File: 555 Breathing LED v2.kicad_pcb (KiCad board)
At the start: 2 copper layers, 80.8 x 35.6 mm, 17 parts, among them Q1 PN2222A, SW1 SW_SPDT, U1 LMC555xN

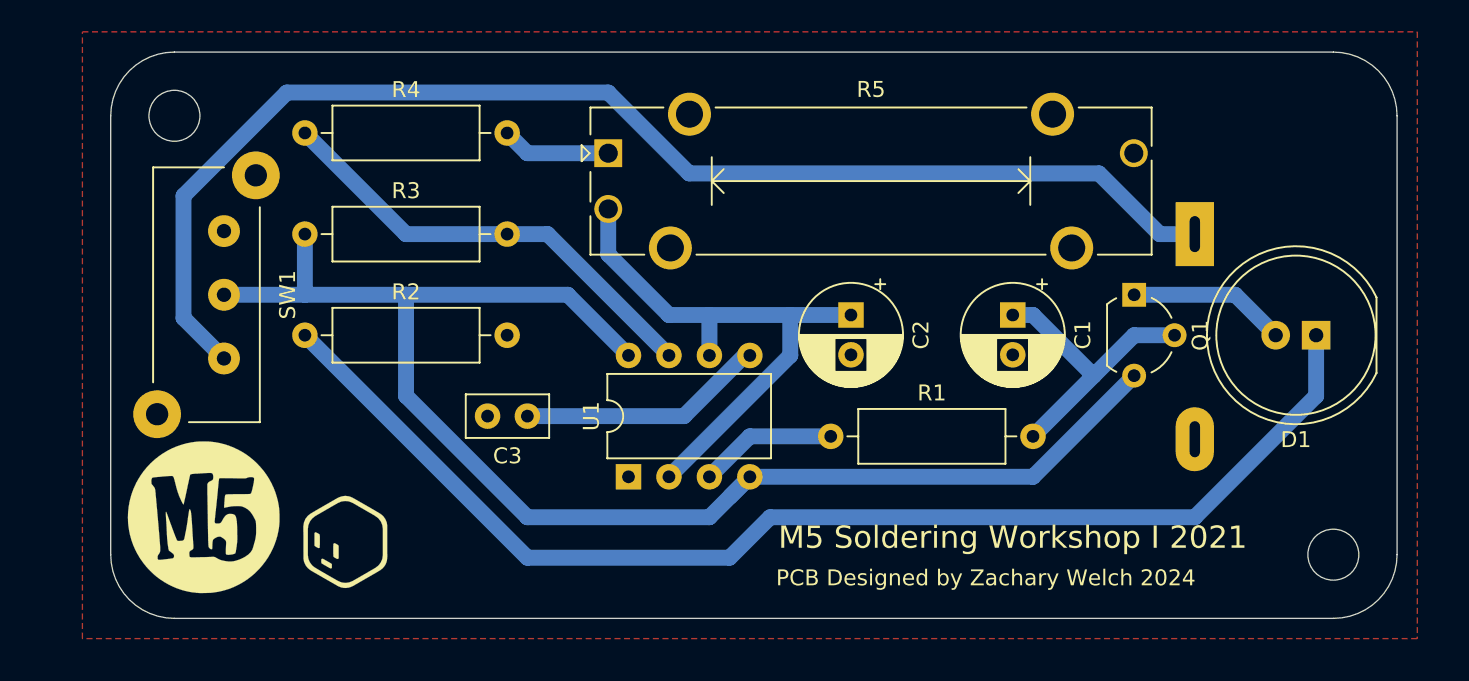
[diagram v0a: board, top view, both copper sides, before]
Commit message: Updated, epic fortnite
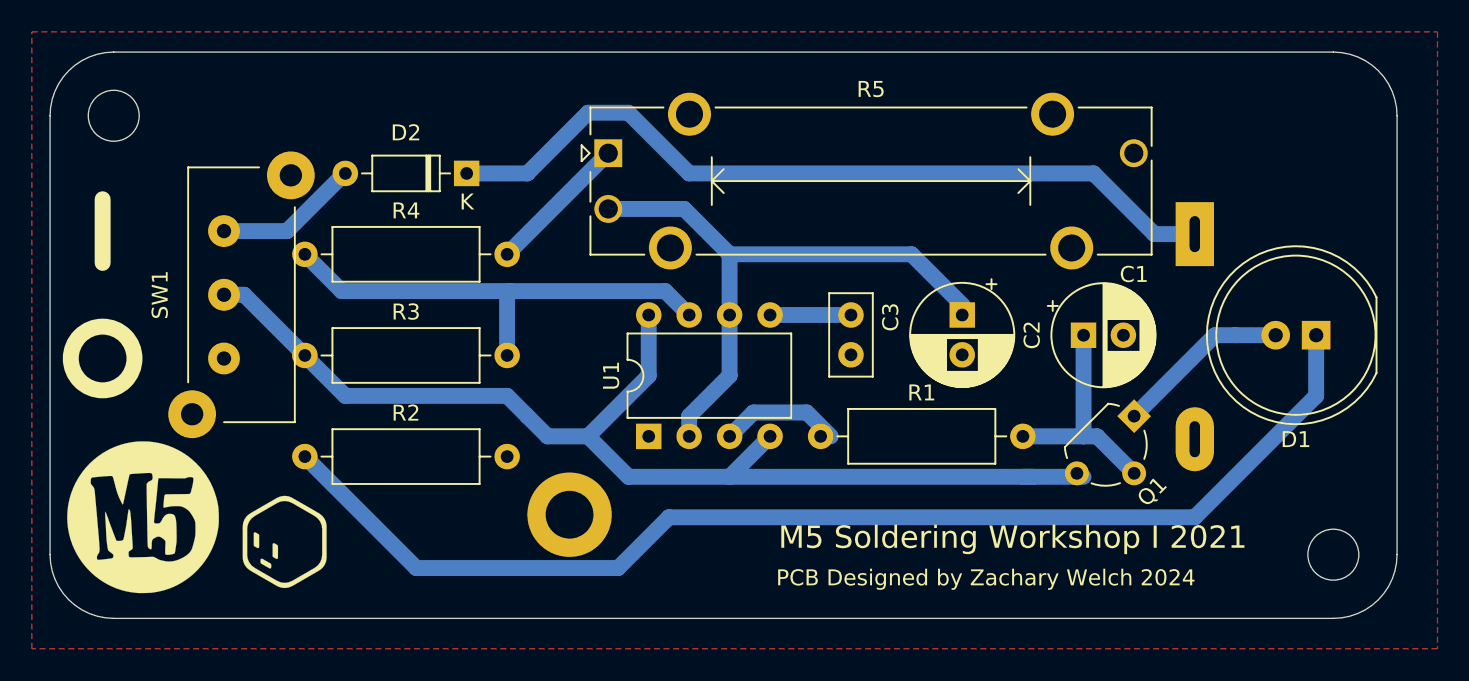
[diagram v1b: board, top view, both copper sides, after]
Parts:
- added D2: 1N4148, Diode_THT:D_DO-35_SOD27_P7.62mm_Horizontal, F.Cu at (76.2, 73.7)
- added REF**: Switch Indicator, Local:Switch Indicator, F.Cu at (53.3, 81.3)
- added REF**: Standoff_M2x0.4, Local:Standoff_M2x0.4, F.Cu at (82.7, 95.1)
- BT1: footprint 555-Breathing-LED-v2:BatteryHolder_MPD_BA9VPC_1xPP3noholes -> Local:BatteryHolder_MPD_BA9VPC_1xPP3noholes
- R2: value 220 -> 100
- moved C3 21.3 mm to (100.3, 82.5), turned to 270 degrees
- moved Q1 7.62 mm to (118.1, 88.9), turned to 225 degrees
- moved R2 7.62 mm to (66.0, 91.4)
- moved R3 7.62 mm to (66.0, 85.1)
- moved R4 7.62 mm to (66.0, 78.7)
- moved C2 6.98 mm to (107.3, 82.5)
- moved C1 4.62 mm to (114.9, 83.8), turned to 0 degrees
- moved ? 3.81 mm to (64.8, 96.8)
- moved ? 3.81 mm to (55.9, 95.2)
- moved REF** 3.81 mm to (61.0, 69.8)
- moved U1 2.84 mm to (87.6, 90.2)
- moved R1 0.64 mm to (98.4, 90.2)
- turned SW1 to 90 degrees
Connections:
- SW1 pad 1: Net-(BT1-Pad1) -> Net-(D2-Pad2)
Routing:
- net Net-(BT1-Pad1): track 81.1 -> 50.5 mm
- net VCC: track 91.5 -> 72.1 mm
- net Net-(C3-Pad1): track 15.5 -> 5.08 mm
- net Net-(D2-Pad2): track 0.00 -> 9.12 mm
- net Net-(C1-Pad1): track 18.2 -> 14.3 mm
- net Net-(D1-Pad1): track 77.3 -> 74.7 mm
- net Net-(C2-Pad1): track 35.5 -> 37.8 mm
- net Net-(R4-Pad2): track 6.88 -> 8.98 mm
- net Net-(R3-Pad2): track 28.6 -> 29.8 mm
- net out: track 8.67 -> 7.59 mm
- net Net-(D1-Pad2): track 9.94 -> 11.0 mm
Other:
- board size 80.8 x 35.6 mm -> 84.6 x 35.6 mm
